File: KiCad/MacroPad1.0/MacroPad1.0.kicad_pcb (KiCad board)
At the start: 2 copper layers, 81 x 41.3 mm, 28 parts, among them SW1 SW_Push, U1 ATmega32U4-A, Y1 16MHz

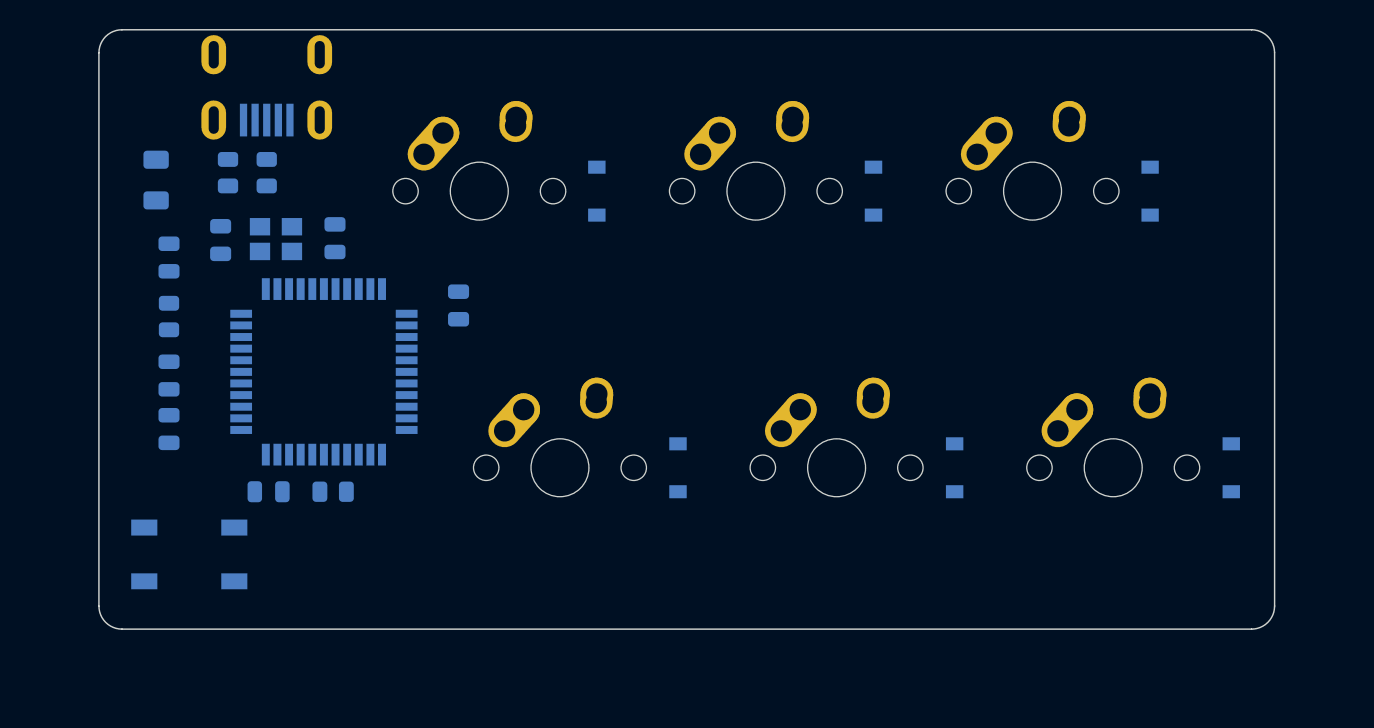
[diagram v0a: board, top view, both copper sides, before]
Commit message: PCB traces complete
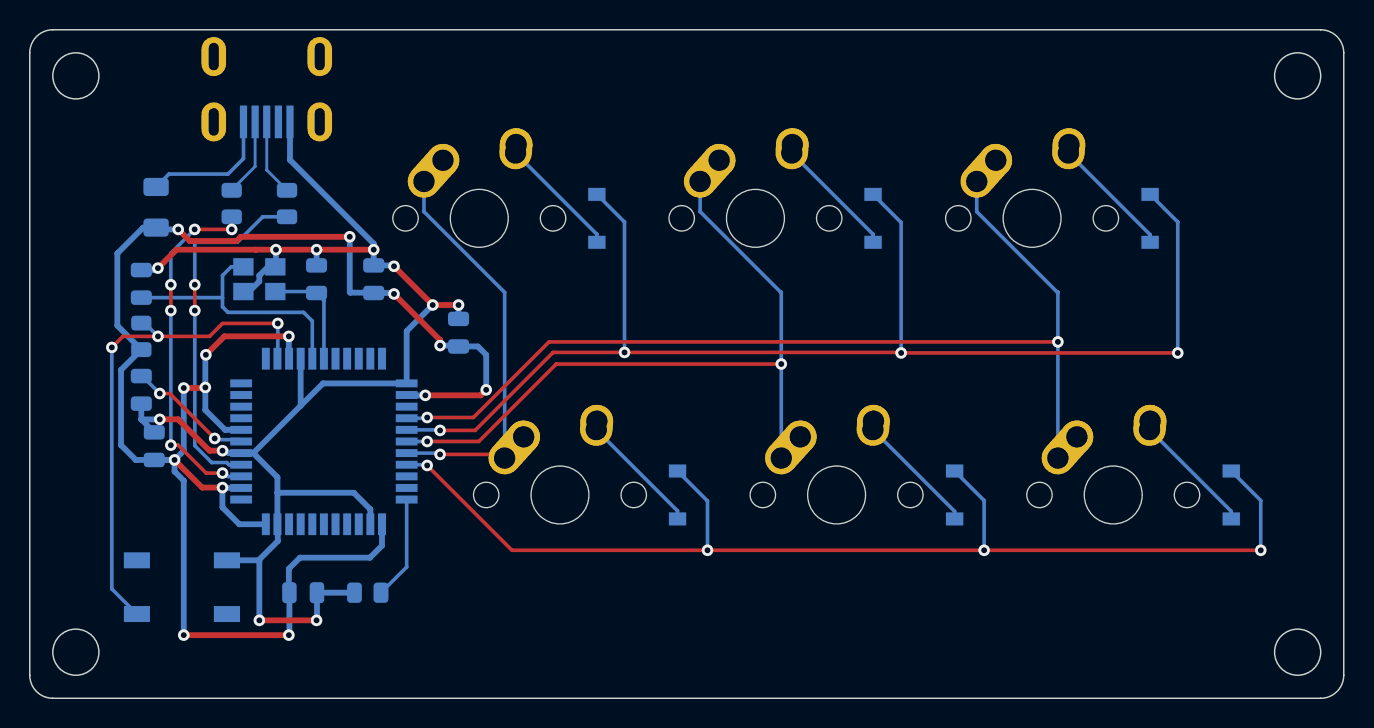
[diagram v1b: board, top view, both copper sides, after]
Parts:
- moved MX2 24.9 mm to (101.6, 103.5)
- moved D2 24.9 mm to (109.7, 103.5)
- moved D5 21.8 mm to (142.2, 84.4)
- moved MX5 21.8 mm to (134.1, 84.4)
- moved D3 19.2 mm to (123.2, 84.4)
- moved MX3 19.2 mm to (115.1, 84.4)
- moved MX4 19.1 mm to (120.7, 103.5)
- moved D4 19.1 mm to (128.8, 103.5)
- moved R4 7.35 mm to (88.4, 110.2)
- moved C5 7.35 mm to (83.9, 110.2)
- moved C2 7.13 mm to (84.8, 88.6)
- moved U1 4.79 mm to (85.3, 99.8)
- moved C1 3.88 mm to (88.8, 88.6)
- moved Y1 2.99 mm to (80.9, 88.6)
- moved C3 2.63 mm to (72.8, 88.9)
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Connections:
- U1 pad 26: unconnected-(U1-Pad26) -> Col2
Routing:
- net +5V: track 0.00 -> 123.3 mm, vias 0 -> 14
- net GND: track 0.00 -> 106.5 mm, vias 0 -> 11
- net Row0: track 0.00 -> 90.5 mm, vias 0 -> 4
- net Row1: track 0.00 -> 80.2 mm, vias 0 -> 4
- net Col2: track 0.00 -> 68.4 mm, vias 0 -> 2
- net Col1: track 0.00 -> 49.4 mm, vias 0 -> 2
- net Net-(R3-Pad1): track 0.00 -> 35.1 mm, vias 0 -> 3
- net Col0: track 0.00 -> 28.2 mm, vias 0 -> 1
- net Net-(R2-Pad2): track 0.00 -> 24.8 mm, vias 0 -> 2
- net Net-(R1-Pad2): track 0.00 -> 24.7 mm, vias 0 -> 6
- net Net-(C3-Pad1): track 0.00 -> 18.6 mm
- net VCC: track 0.00 -> 9.35 mm
- net Net-(C7-Pad1): track 0.00 -> 8.74 mm, vias 0 -> 2
- net Net-(D6-Pad2): track 0.00 -> 8.48 mm
- net Net-(D5-Pad2): track 0.00 -> 8.48 mm
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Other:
- board size 81 x 41.3 mm -> 90.5 x 46 mm
